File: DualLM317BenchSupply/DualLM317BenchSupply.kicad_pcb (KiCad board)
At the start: 2 copper layers, 81.3 x 68.6 mm, 40 parts, among them CON101 BARREL_JACK, P103 CONN_1, P104 CONN_1, SW101 SPDT, SW102 SPDT, SW103 SPDT, SW201 SP6T, U101 7805, U102 LM317, U103 LM317

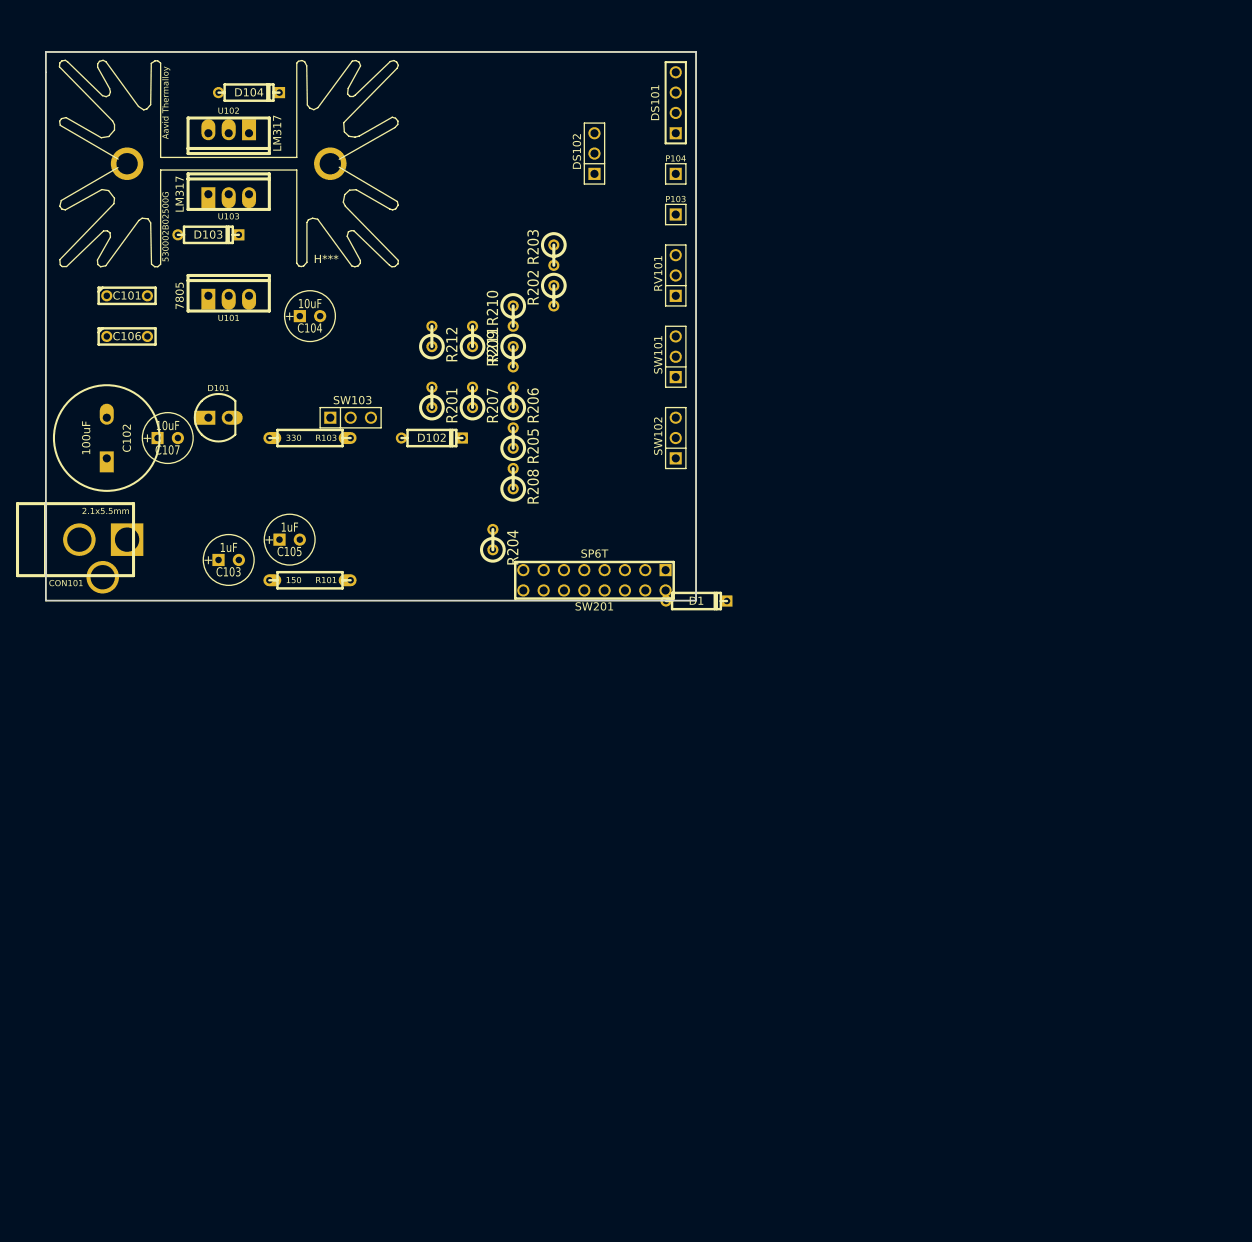
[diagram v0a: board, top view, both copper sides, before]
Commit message: working on board layout
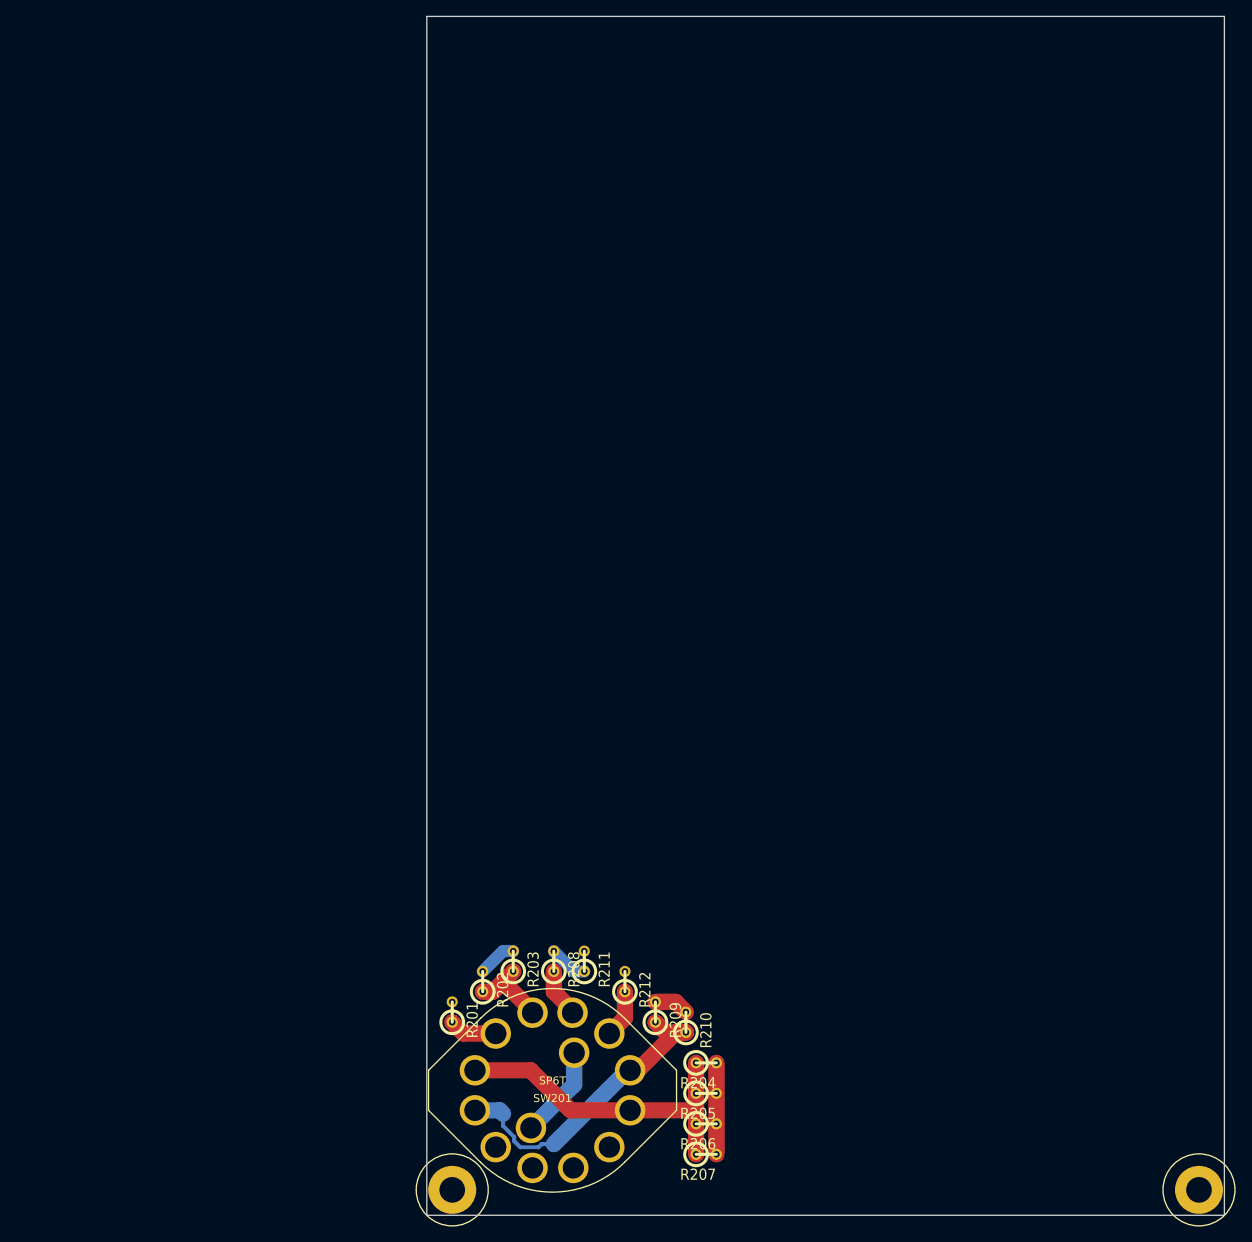
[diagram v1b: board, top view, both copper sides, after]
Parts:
- removed C101, C106: 0.1uF, C2
- removed C102: 100uF, ELCAP_2_52_V
- removed C103, C105: 1uF, C1V7
- removed C104, C107: 10uF, C1V7
- removed CON101: BARREL_JACK, BARREL_JACK_21x55
- removed D1, D102, D103, D104: 1N4148, D3
- removed D101: LED, LED_5MM
- removed DS101: AMMETER, PIN_ARRAY_4x1
- removed DS102: VOLTMETER, PIN_ARRAY_3X1
- removed the H*** at (124.5, 133.3)
- removed P103, P104: CONN_1, PIN_ARRAY_1
- removed R101: 150, R_AXIAL_0W25
- removed R103: 330, R_AXIAL_0W25
- removed RV101: 5k, PIN_ARRAY_3X1
- removed SW101, SW102, SW103: SPDT, PIN_ARRAY_3X1
- removed U101: 7805, TO-220_V_069B
- removed U102, U103: LM317, TO-220_V_069B
- added H***: Val**, hole_M3, F.Cu at (139.7, 261.6)
- added H***: Val**, hole_M3, F.Cu at (233.0, 261.6)
- SW201: footprint pin_array_8x2 -> G3SR022-R
- moved R207 99.0 mm to (171.4, 257.2), turned to 0 degrees
- moved R206 94.0 mm to (171.4, 253.4), turned to 0 degrees
- moved R210 90.9 mm to (168.9, 240.7), turned to 90 degrees
- moved R203 88.4 mm to (147.3, 233.0), turned to 90 degrees
- moved R202 86.2 mm to (143.5, 235.6), turned to 90 degrees
- moved R205 85.4 mm to (171.4, 249.6), turned to 0 degrees
- moved R212 84.2 mm to (161.3, 235.6)
- moved R209 83.8 mm to (165.1, 239.4), turned to 90 degrees
- moved R211 79.3 mm to (156.2, 233.0)
- moved R201 76.9 mm to (139.7, 239.4)
- moved R204 70.6 mm to (171.4, 245.7), turned to 0 degrees
- moved R208 60.5 mm to (152.4, 233.0)
- moved SW201 59.1 mm to (154.9, 244.5), turned to 0 degrees
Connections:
- R204 pad 1: N-0000019 -> N-0000015
- R204 pad 2: N-0000018 -> /current_limit_r/OUT
- R205 pad 1: N-0000018 -> N-0000015
- R206 pad 1: N-0000020 -> N-0000015
- R207 pad 1: N-0000017 (its old number) -> N-0000015
- R208 pad 1: N-0000017 (its old number) -> N-0000020
- R208 pad 2: /current_limit_r/OUT -> N-0000016
- R209 pad 1: N-0000021 (its old number) -> N-0000019
- R210 pad 1: N-0000021 (its old number) -> N-0000019
- R211 pad 1: N-0000021 (its old number) -> N-0000016
- R212 pad 1: N-0000021 (its old number) -> N-0000018
- SW201 pad 4: N-0000019 -> N-0000020
- SW201 pad 5: N-0000020 -> N-0000018
- SW201 pad 6: N-0000017 (its old number) -> N-0000019
- SW201 pad 7: N-0000021 (its old number) -> N-0000015
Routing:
- net N-0000015: track 0.00 -> 42.6 mm
- net N-0000019: track 0.00 -> 39.8 mm
- net /current_limit_r/OUT: track 0.00 -> 20.6 mm
- net /current_limit_r/IN: track 0.00 -> 11.6 mm
- net N-0000017: track 0.00 -> 10.3 mm
- net N-0000020: track 0.00 -> 6.13 mm
- net N-0000018: track 0.00 -> 6.03 mm
- net N-0000021: track 0.00 -> 6.02 mm
- net N-0000016: track 0.00 -> 4.86 mm
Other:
- board size 81.3 x 68.6 mm -> 99.7 x 149.9 mm
